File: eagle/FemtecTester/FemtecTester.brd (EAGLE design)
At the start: 72.1 x 49.5 mm, 54 parts, among them IC1 FT232RL, IC2 ATMEGA644A, K1 AQY212, K2 AQY212

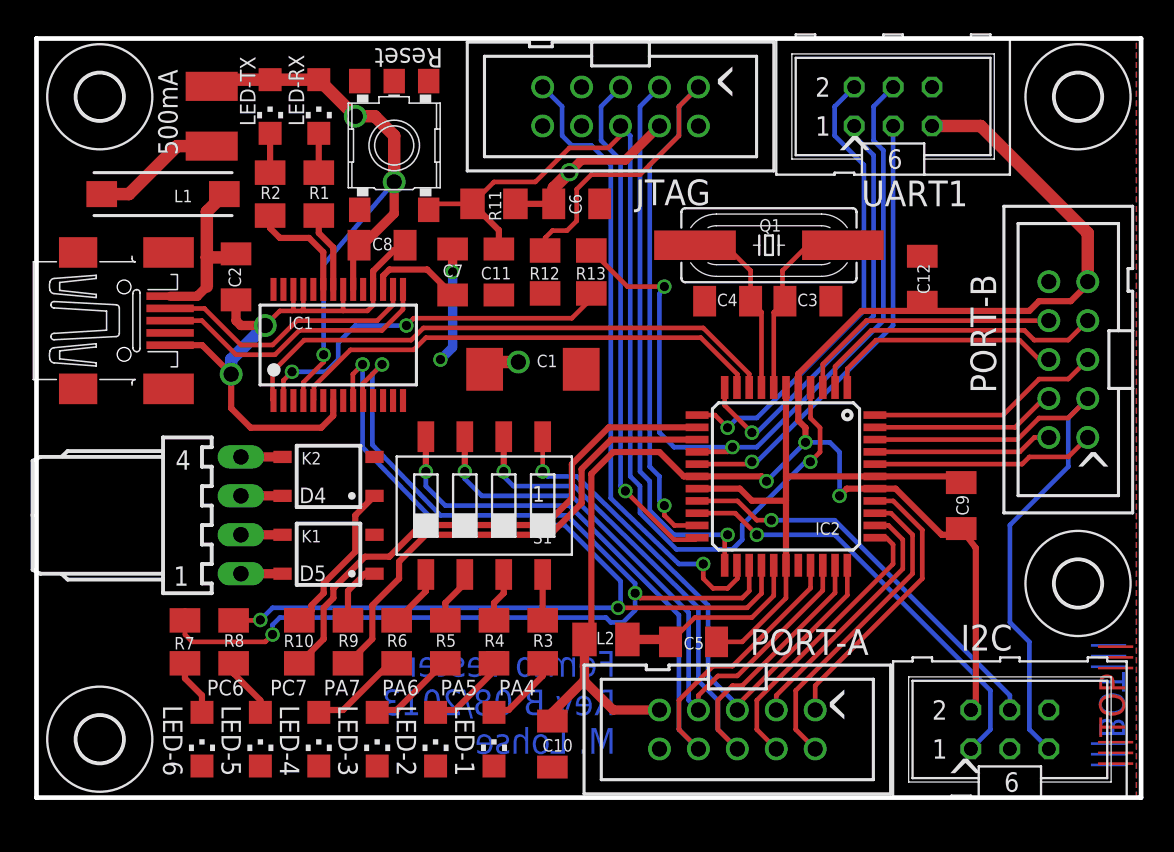
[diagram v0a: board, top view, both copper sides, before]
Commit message: update FemtoTester eagle files (rev. B)
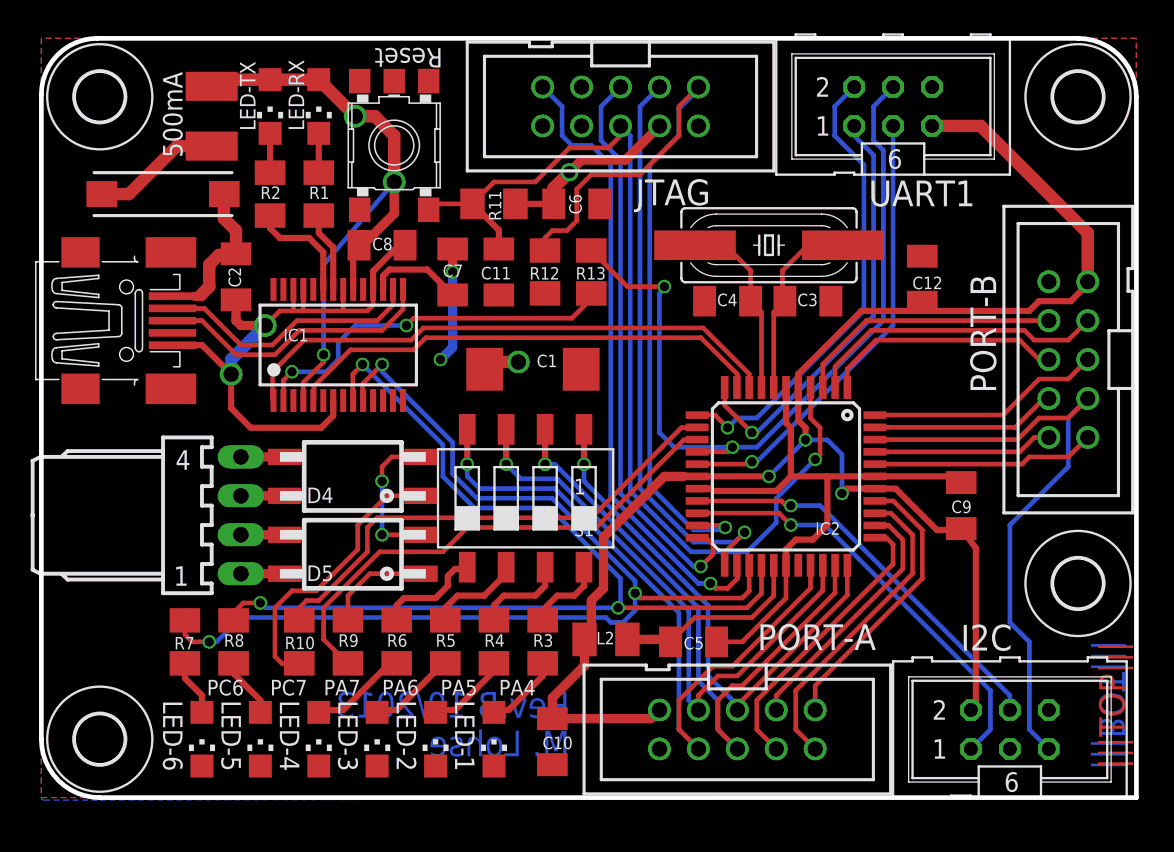
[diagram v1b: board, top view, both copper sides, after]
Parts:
- K1, K2: device relay:SOP04 -> tpv:SMD-DIP04
- U$1, U$2, U$3, U$4: device holes:3,0 -> holes:3,2
- moved S1 2.74 mm to (31.9, 19.5)
- moved K1 1.59 mm to (20.6, 15.9), turned to 180 degrees
- moved K2 1.59 mm to (20.6, 21.0), turned to 180 degrees
- moved USB 0.16 mm to (5.87, 31.1)
- moved C10 0.16 mm to (33.7, 3.65)
- turned R10 to 270 degrees
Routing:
- net GND: track 85.3 -> 97.0 mm, vias 4 -> 6
- net N$29: track 10.2 -> 18.4 mm
- net TMS: track 33.6 -> 38.0 mm
- net VCC: track 167.1 -> 163.2 mm
- net TCK: track 49.3 -> 52.6 mm
- net N$15: track 3.78 -> 6.99 mm
- net N$28: track 4.12 -> 6.97 mm
- net DCD: track 73.2 -> 70.4 mm
- net N$9: track 3.26 -> 6.06 mm
- net A6: track 41.1 -> 38.4 mm
- net A5: track 45.1 -> 42.5 mm
- net N$14: track 3.52 -> 6.14 mm
- net N$20: track 35.2 -> 32.6 mm
- net A7: track 49.3 -> 46.8 mm
- net A4: track 37.1 -> 34.9 mm
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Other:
- board size 72.1 x 49.5 mm -> 71.4 x 49.5 mm
- board text added: "1"
- board text added: "5"
- board text added: "9"
- board text added: "Rev.B 10/2013 M. Lohse"
- board text removed: "Femto Tester Rev.B 08/2013 M. Lohse"
- board text removed: "^"
